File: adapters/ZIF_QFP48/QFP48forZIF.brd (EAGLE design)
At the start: 54 x 59.7 mm, 8 parts, among them J1 0

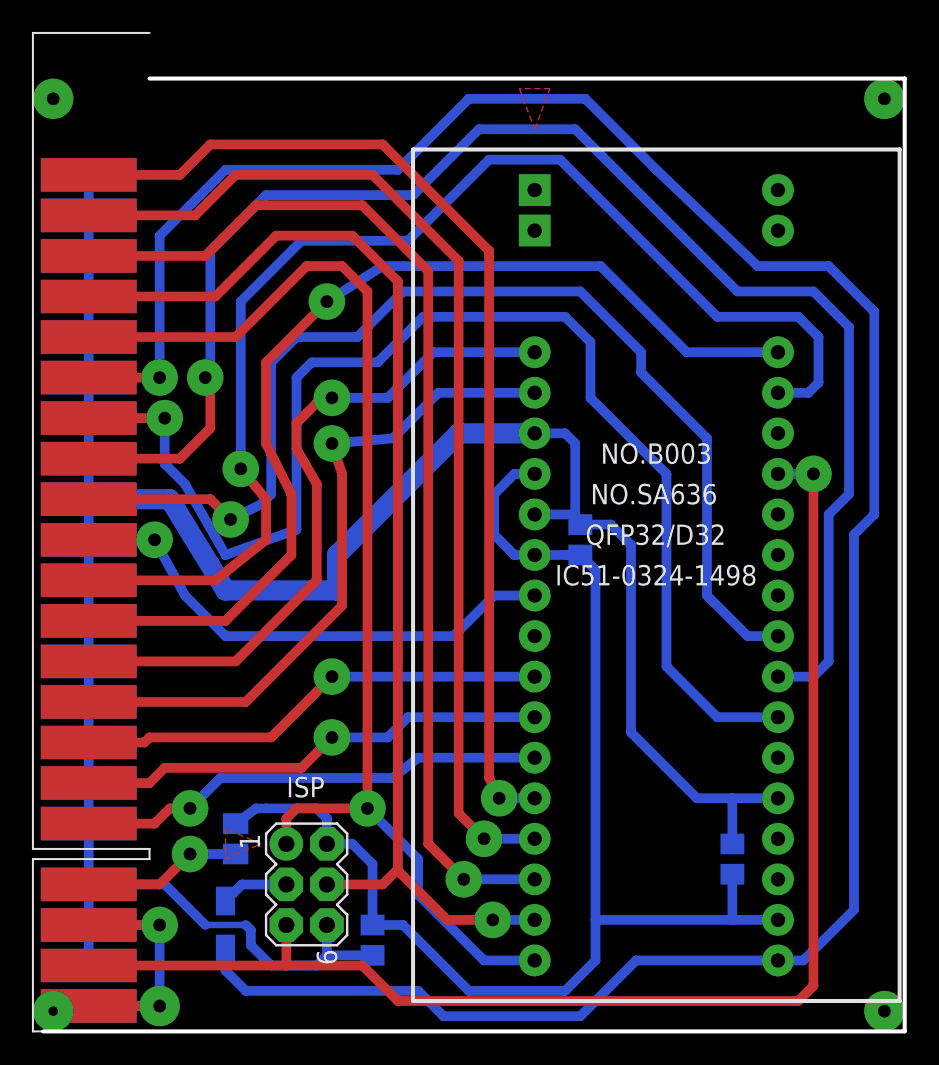
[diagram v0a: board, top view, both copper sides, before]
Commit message: rename adapter
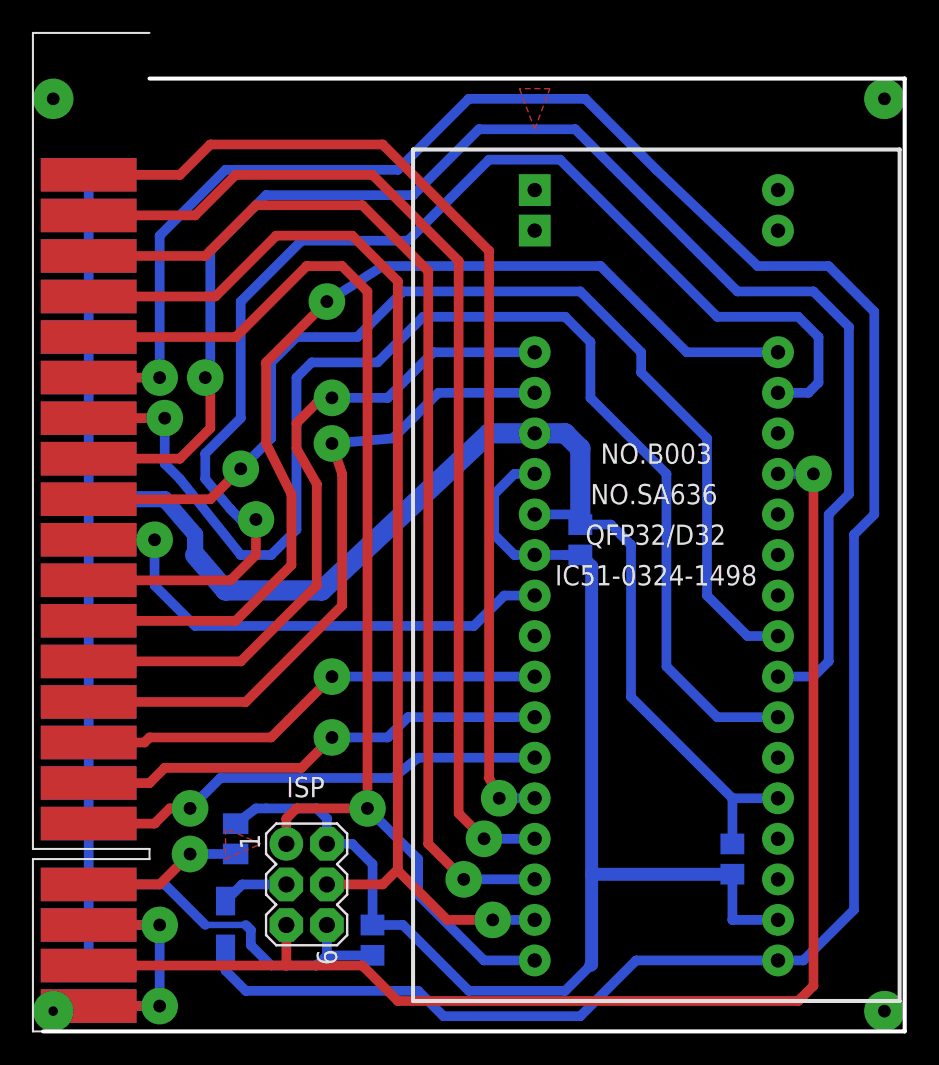
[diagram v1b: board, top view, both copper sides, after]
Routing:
- net BS2: track 69.7 -> 66.8 mm
- net GND: track 171.3 -> 169.0 mm
- net R/B: track 77.6 -> 79.9 mm
- net XTAL1: track 32.1 -> 32.6 mm
